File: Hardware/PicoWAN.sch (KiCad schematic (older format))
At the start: 49 parts, among them J1 Battery, J2 SWD, J3 Conn_left, J4 Conn_right, P1 USB_C_Plug_USB2.0, Q1 DMG3415U-7, SW1 BOOT, SW2 RESET, U1 AP2112K-3.3, U2 RP2040, U3 MCP73831-2-OT, U4 W25Q16JV, U5 RFM95W-868S2, Y2 12Mhz

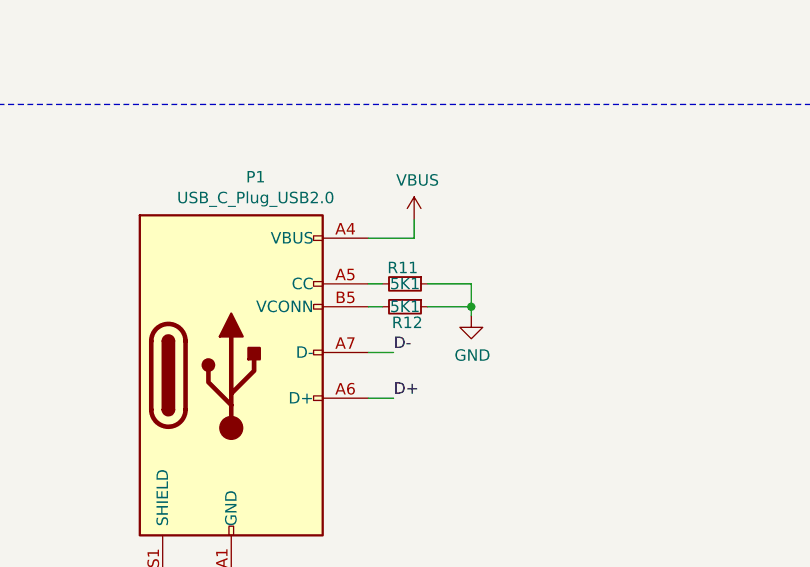
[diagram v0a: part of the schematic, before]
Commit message: Add_BOM
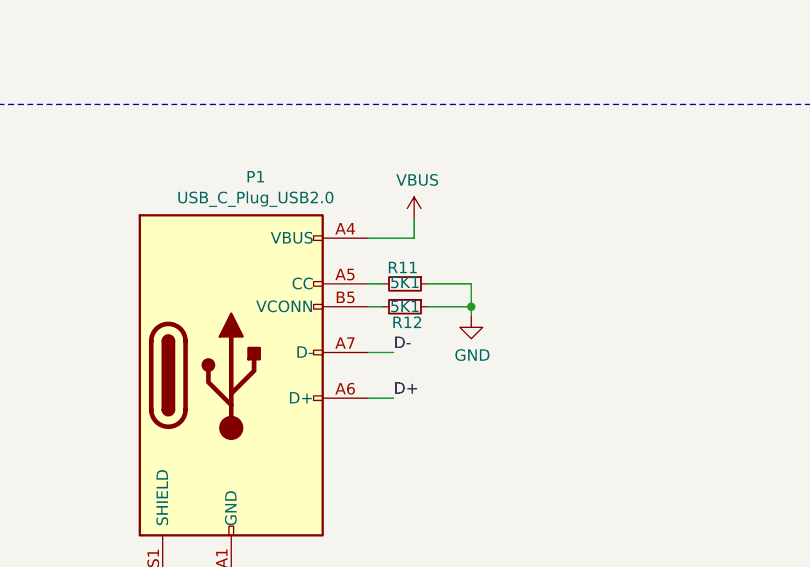
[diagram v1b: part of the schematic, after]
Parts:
- AE1: LCSC# (none) -> C88373; manf# (none) -> U.FL-R-SMT-1(10)
- C1, C2: LCSC# (none) -> C482483; manf# (none) -> HGC0402G0220J500NTEJ
- C10, C11, C12, C13, C14, C15, C18, C19, C4, C6, C9: LCSC# (none) -> C106209; manf# (none) -> CC0402ZRY5V7BB104
- C16, C17: LCSC# (none) -> C15525; manf# TCSOM1A106M8R-ZM1 -> CL05A106MQ5NUNC
- C3, C7: LCSC# (none) -> C15684; manf# (none) -> GRM155R60J105KE19D
- C5: LCSC# (none) -> C307423; manf# CL10A475KA8NQNC -> CL05A475MQ5NRNC
- C8: LCSC# (none) -> C15684; manf# CL10A105KA8NNNC -> GRM155R60J105KE19D
- D1: LCSC# (none) -> C223608; manf# NRVB120VLSFT1G -> MBR120VLSFT1G
- D2: LCSC# (none) -> C205443; manf# 150080GS75000 -> ORH-G36G
- D3: LCSC# (none) -> C118330; manf# (none) -> D-060306R1/SS2/L
- J1: manf# AR0165 -> (none)
- P1: LCSC# (none) -> C393939; manf# (none) -> TYPE-C16PIN
- Q1: LCSC# (none) -> C96616; manf# (none) -> DMG3415U-7
- R1: LCSC# (none) -> C15458; manf# CRCW0603100KFKEAC -> 0603WAJ0104T5E
- R10, R3, R8: LCSC# (none) -> C140214; manf# (none) -> RC-02W103JT
- R11, R12: LCSC# (none) -> C131715; manf# (none) -> RK73B1JTTD512J
- R2, R9: LCSC# (none) -> C384390; manf# (none) -> WR04X102JTL
- R4, R5: LCSC# (none) -> C384351; manf# (none) -> WR04X270JTL
- R6: LCSC# (none) -> C25590; manf# CRCW06032K00FKEAC -> 0603WAJ0202T5E
- R7: LCSC# (none) -> C384390; manf# CRCW06031K00FKEAC -> WR04X102JTL
- SW1, SW2: LCSC# (none) -> C455281; manf# (none) -> TS-1088R-02526
- U1: LCSC# (none) -> C51118; manf# (none) -> AP2112K-3.3TRG1
- U3: LCSC# (none) -> C424093
- U4: LCSC# (none) -> 454-W25Q16JVUXIQTR
- Y2: LCSC# (none) -> C709001; manf# C709001 -> CM4012M00020T8188026
